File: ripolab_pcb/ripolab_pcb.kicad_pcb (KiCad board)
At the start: 2 copper layers, 94.7 x 83.2 mm, 38 parts, among them J1 Conn_01x02, SW1 SPDT, U1 ESP-12, U2 SPX3819M5-L-3-3

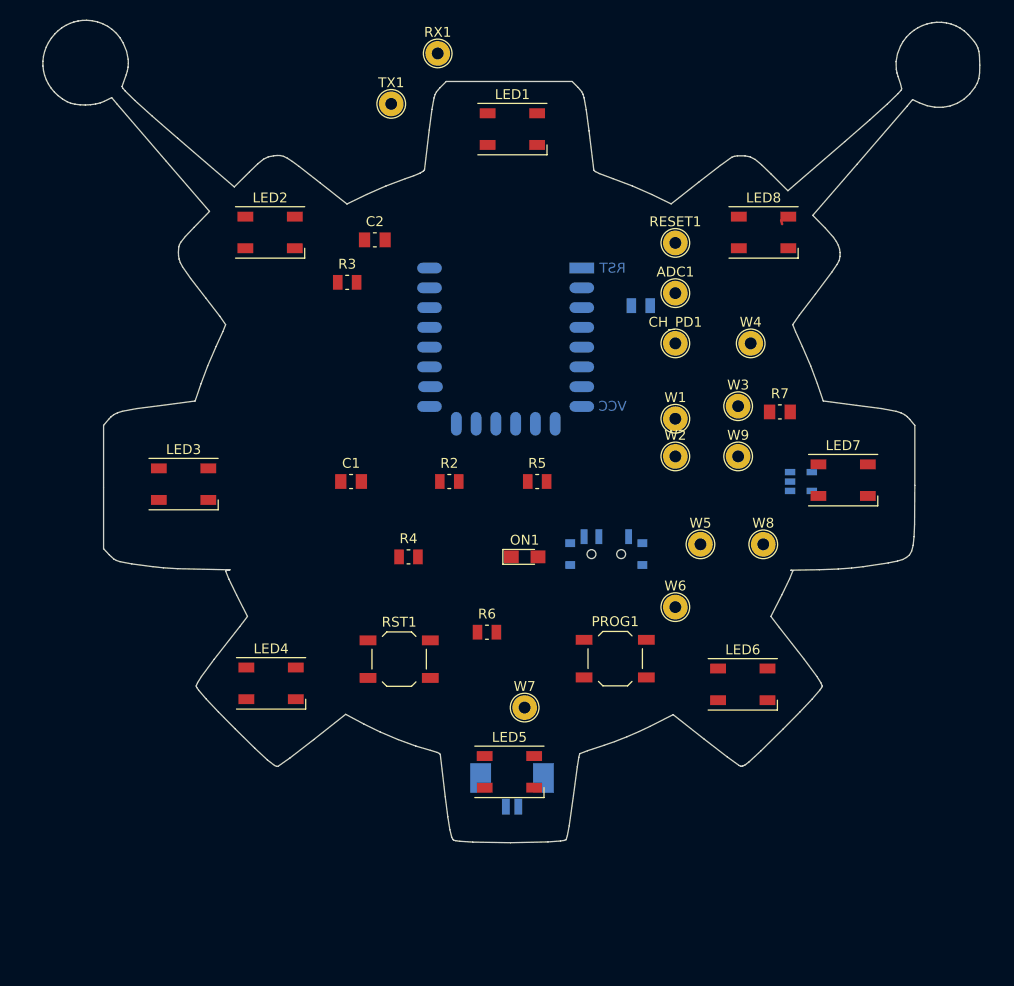
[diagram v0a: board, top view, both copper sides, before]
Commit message: badge ripolab v1
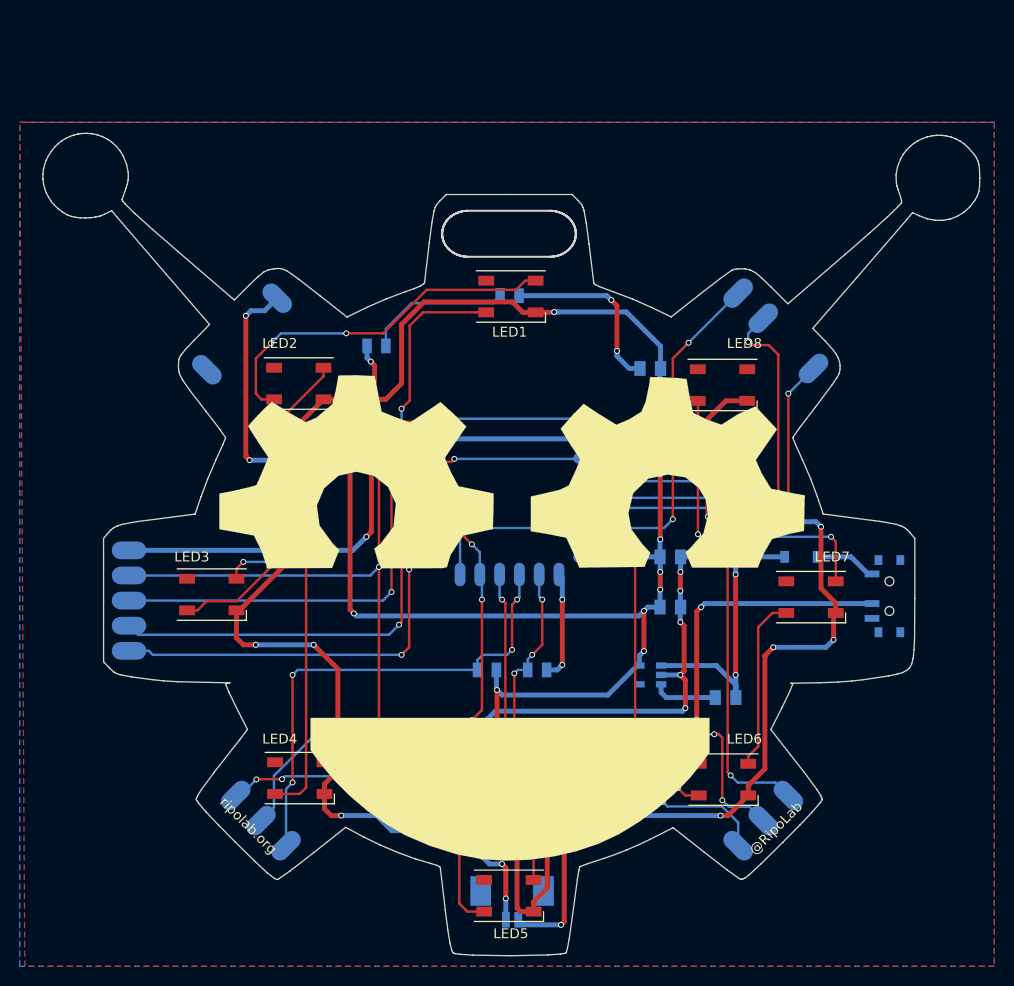
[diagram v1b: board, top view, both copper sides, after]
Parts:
- removed ADC1: ADC, TestPoint:TestPoint_THTPad_D2.5mm_Drill1.2mm
- removed CH_PD1: CH_PD, TestPoint:TestPoint_THTPad_D2.5mm_Drill1.2mm
- removed RESET1, W1, W2, W3, W4, W5, W6, W7, W8, W9: TEST_1P, TestPoint:TestPoint_THTPad_D2.5mm_Drill1.2mm
- removed RX1: RX, TestPoint:TestPoint_THTPad_D2.5mm_Drill1.2mm
- removed TX1: TX, TestPoint:TestPoint_THTPad_D2.5mm_Drill1.2mm
- added ADC_1: ADC, ripolab_pcb:TestPad, B.Cu at (108.6, 92.0)
- added C3: 10nF, Capacitor_SMD:C_0805_2012Metric_Pad1.15x1.50mm_HandSolder, B.Cu at (163.3, 97.8)
- added C4: 47uF, Capacitor_SMD:C_0805_2012Metric_Pad1.15x1.50mm_HandSolder, B.Cu at (163.3, 92.7)
- added CH_PD_1: CH_PD, ripolab_pcb:TestPad, B.Cu at (108.6, 97.1)
- added D1: D_Schottky_ALT, Diode_SMD:D_SOD-123, B.Cu at (176.5, 92.7)
- added GND_1: GND, ripolab_pcb:TestPad, B.Cu at (116.5, 73.8)
- added GPIO0: TEST_1P, ripolab_pcb:TestPad, B.Cu at (119.4, 116.8)
- added GPIO12: TEST_1P, ripolab_pcb:TestPad, B.Cu at (177.8, 73.7)
- added GPIO13: TEST_1P, ripolab_pcb:TestPad, B.Cu at (170.2, 121.9)
- added GPIO14: TEST_1P, ripolab_pcb:TestPad, B.Cu at (172.7, 68.6)
- added GPIO15: TEST_1P, ripolab_pcb:TestPad, B.Cu at (172.7, 119.4)
- added GPIO16: TEST_1P, ripolab_pcb:TestPad, B.Cu at (175.3, 116.8)
- added GPIO2: TEST_1P, ripolab_pcb:TestPad, B.Cu at (124.5, 121.9)
- added GPIO4: TEST_1P, ripolab_pcb:TestPad, B.Cu at (121.9, 119.4)
- added GPIO5: TEST_1P, ripolab_pcb:TestPad, B.Cu at (170.2, 66.0)
- added REF**: KiCad-Logo2_6mm_SilkScreen, Symbol:KiCad-Logo2_6mm_SilkScreen, B.Cu at (128.5, 77.5)
- added REF**: OSHW-Logo2_9.8x8mm_SilkScreen, Symbol:OSHW-Logo2_9.8x8mm_SilkScreen, B.Cu at (125.7, 87.4)
- added RST_1: TEST_1P, ripolab_pcb:TestPad, B.Cu at (108.6, 94.6)
- added RX_1: RX, ripolab_pcb:TestPad, B.Cu at (108.6, 102.2)
- added TX_1: TX, ripolab_pcb:TestPad, B.Cu at (108.6, 99.7)
- added VCC_1: TEST_VCC, ripolab_pcb:TestPad, B.Cu at (123.6, 66.5)
- added svg2mod: G***, ripolab_pcb:logo_ripolab_12x14mm, B.Cu at (127.8, 101.3)
- added svg2mod: G***, ripolab_pcb:logo_pcb_cara, F.Cu at (147.3, 99.1)
- C1: value 10nF -> 47uF; moved to B.Cu
- C2: value C -> 100nF; moved to B.Cu
- ON1: footprint LEDs:LED_0805_HandSoldering -> LED_SMD:LED_0805_2012Metric; moved to B.Cu
- PROG1, R2, R3, R4, R5, R6, RST1: moved to B.Cu
- R7: value R -> 10K; moved to B.Cu
- moved C2 47.8 mm to (168.9, 92.7), turned to 180 degrees
- moved R3 43.6 mm to (149.9, 104.1), turned to 180 degrees
- moved C1 32.3 mm to (161.3, 73.7)
- moved R6 31.0 mm to (133.6, 71.4)
- moved R2 30.0 mm to (149.9, 113.8)
- moved R7 29.4 mm to (168.9, 106.9), turned to 180 degrees
- moved SW1 28.7 mm to (185.2, 96.7), turned to 270 degrees
- moved ON1 26.5 mm to (147.1, 66.3), turned to 180 degrees
- moved U2 24.8 mm to (161.3, 104.6), turned to 180 degrees
- moved R4 22.5 mm to (144.8, 113.8), turned to 180 degrees
- moved R5 19.7 mm to (144.8, 104.1), turned to 180 degrees
- moved LED1 16.9 mm to (147.2, 66.4)
- moved LED8 16.0 mm to (168.6, 75.3)
- moved LED2 15.6 mm to (125.8, 75.2)
- moved R1 15.5 mm to (161.3, 82.8), turned to 180 degrees
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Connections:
- C2 pad 1: VBAT_SW -> Net-(C2-Pad1)
- LED8 pad 4: (no net) -> Net-(LED8-Pad4)
- R7 pad 1: VBAT_SW -> Net-(C2-Pad1)
- SW1 pad 3: (no net) -> Net-(SW1-Pad3)
- U2 pad 1: VBAT_SW -> Net-(C2-Pad1)
- U2 pad 4: (no net) -> Net-(U2-Pad4)
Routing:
- net +3,3V: track 0.00 -> 371.3 mm, vias 0 -> 26
- net GND: track 0.00 -> 93.4 mm, vias 0 -> 13
- net Reset: track 0.00 -> 89.4 mm, vias 0 -> 3
- net GPIO4: track 0.00 -> 82.4 mm, vias 0 -> 5
- net GPIO0: track 0.00 -> 68.1 mm, vias 0 -> 5
- net VBAT: track 0.00 -> 67.4 mm, vias 0 -> 4
- net CH_PD: track 0.00 -> 64.7 mm, vias 0 -> 2
- net ADC: track 0.00 -> 54.3 mm, vias 0 -> 4
- net GPIO5: track 0.00 -> 51.6 mm, vias 0 -> 2
- net GPIO16: track 0.00 -> 51.6 mm, vias 0 -> 2
- net GPIO15: track 0.00 -> 50.3 mm, vias 0 -> 6
- net GPIO2: track 0.00 -> 49.3 mm, vias 0 -> 4
- net GPIO13: track 0.00 -> 44.3 mm, vias 0 -> 2
- net GPIO14: track 0.00 -> 41.0 mm, vias 0 -> 2
- net Rx: track 0.00 -> 40.3 mm, vias 0 -> 2
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- added copper zone on B.Cu, net GND
- added copper zone on F.Cu, net GND
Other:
- outline, holes or cut-outs redrawn
- net class Power added: clearance 0.3, trace_width 0.5, via_dia 0.6, via_drill 0.4
- board text added: "@RipoLab"
- board text added: "ADC"
- board text added: "CH_PD"
- board text added: "ESP8266"
- board text added: "GND"
- board text added: "ON"
- board text added: "PROG/USER"
- board text added: "RESET"
- board text added: "RX"
- board text added: "TX"
- board text added: "ripolab.org"
- board text added: "v1.0 2018"
- board text removed: "*Made on Earth by a Maker with Opensource software chupate esa marciano*"
- board text removed: "RST"
